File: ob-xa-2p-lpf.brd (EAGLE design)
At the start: 162.5 x 79.7 mm, 53 parts, among them IC1 AS3320, IC3 TL082P

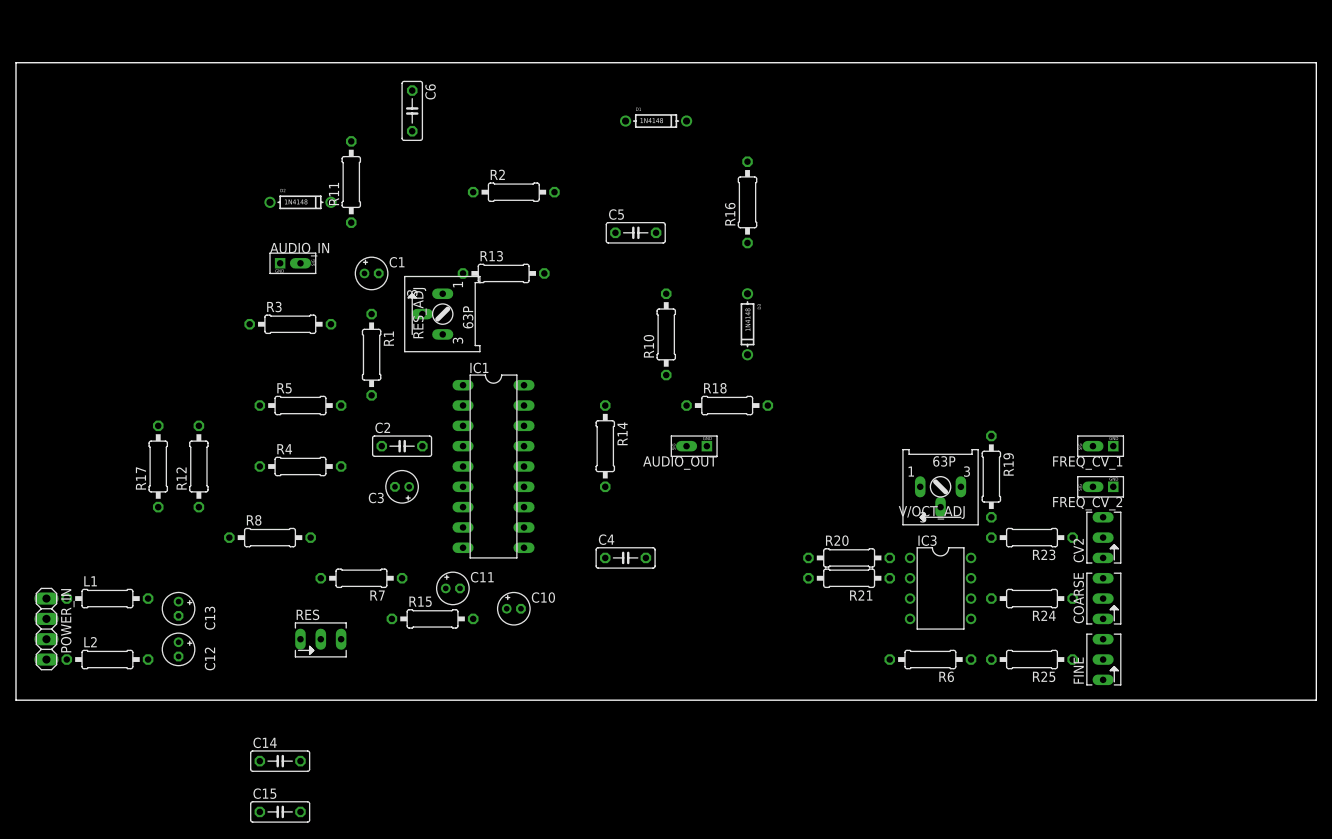
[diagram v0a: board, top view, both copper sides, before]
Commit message: layout everything
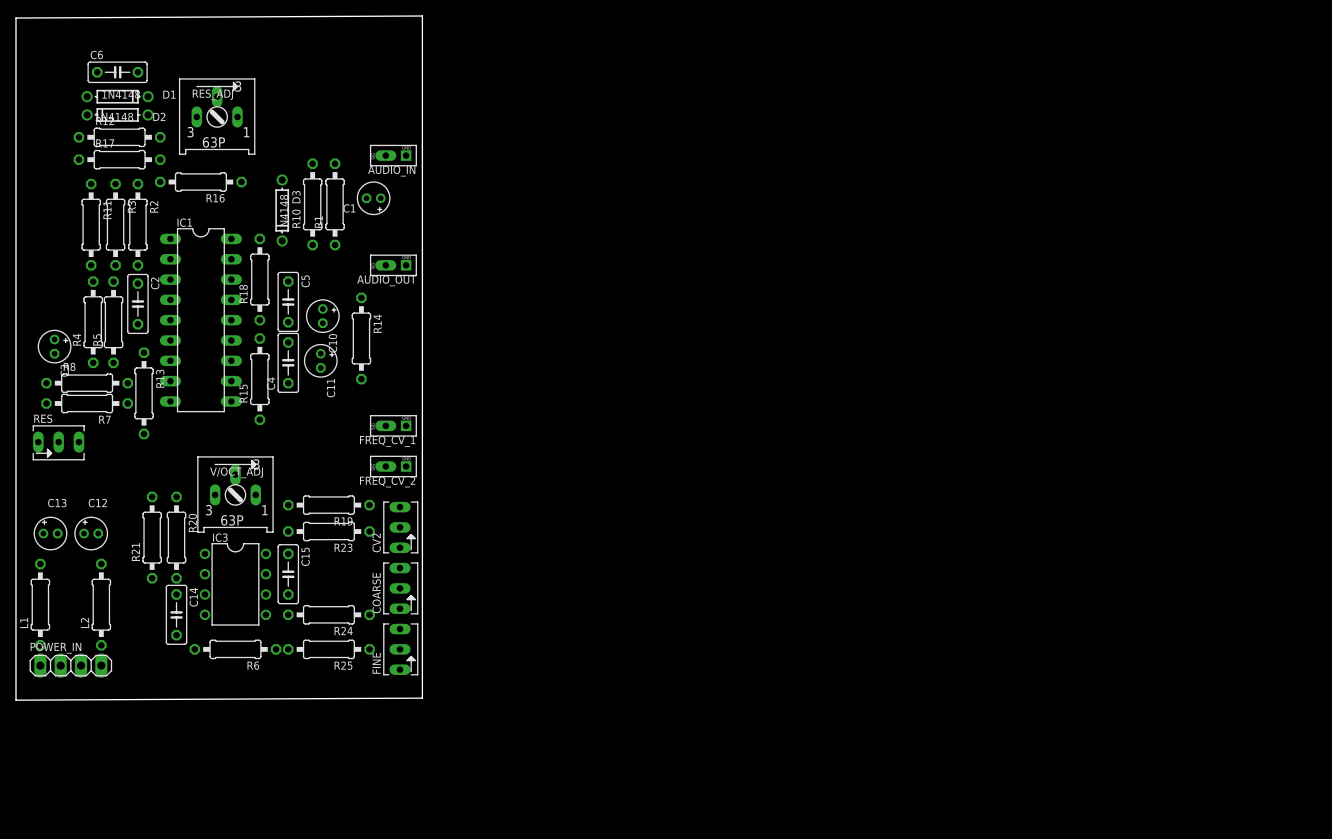
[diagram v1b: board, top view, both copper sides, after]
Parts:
- moved FREQ_CV_1 88.4 mm to (47.5, 35.6)
- moved FREQ_CV_2 88.4 mm to (47.5, 30.5)
- moved V/OCT_ADJ 88.1 mm to (27.4, 25.7), turned to 0 degrees
- moved IC3 88.1 mm to (27.4, 14.5)
- moved R24 87.9 mm to (39.1, 10.7)
- moved R25 87.9 mm to (39.1, 6.35)
- moved COARSE 87.9 mm to (48.0, 14.0)
- moved CV2 87.9 mm to (48.0, 21.6)
- moved FINE 87.9 mm to (48.0, 6.35)
- moved R23 87.9 mm to (39.1, 21.1)
- moved R21 87.3 mm to (17.0, 20.3), turned to 90 degrees
- moved R6 86.9 mm to (27.4, 6.35)
- moved R20 84.1 mm to (20.1, 20.3), turned to 270 degrees
- moved R19 82.9 mm to (39.1, 24.4), turned to 180 degrees
- moved R16 68.4 mm to (23.1, 64.8), turned to 180 degrees
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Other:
- board size 162.5 x 79.7 mm -> 50.8 x 85.5 mm
